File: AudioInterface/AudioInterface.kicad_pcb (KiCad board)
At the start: 2 copper layers, 21 parts, among them J1 Capsule, J2 Set_Gain, J3 Audio_Out, J4 Power, U1 THAT1512, U2 NMA0515SC

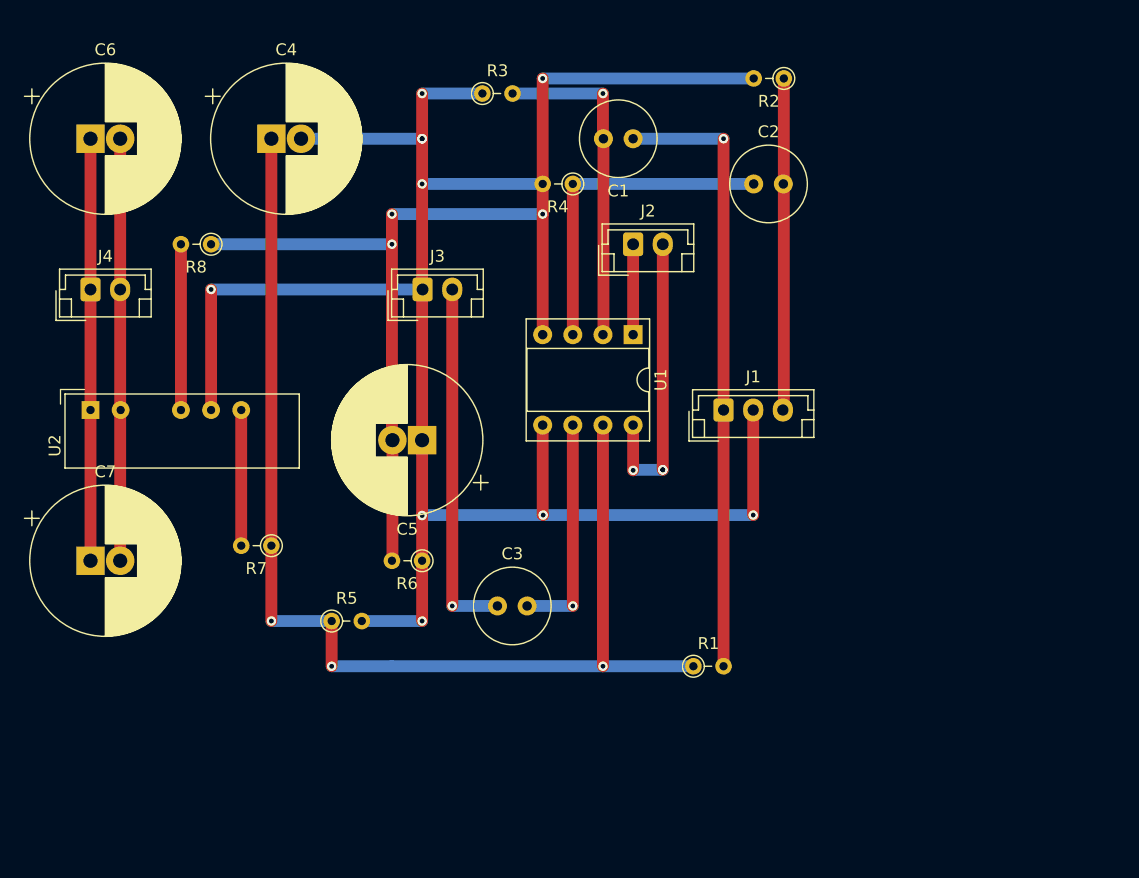
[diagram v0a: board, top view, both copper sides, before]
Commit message: finished pcb
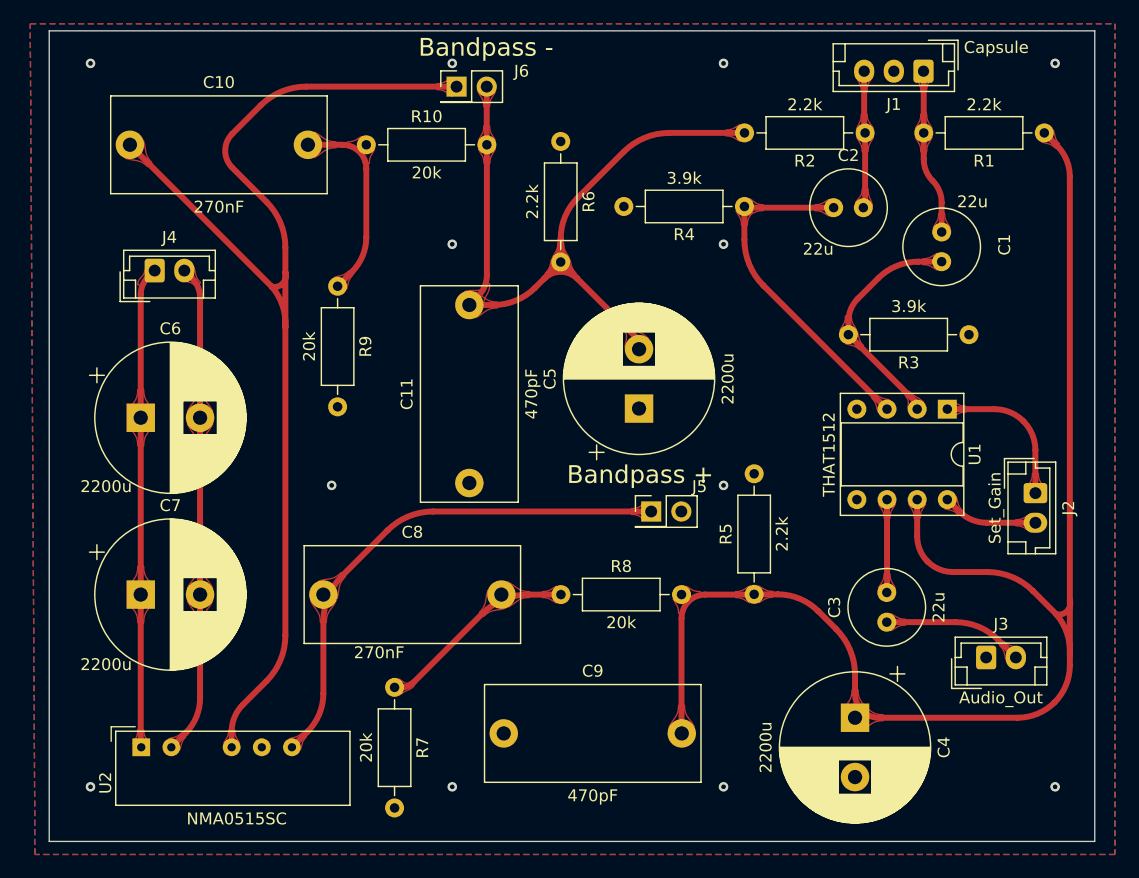
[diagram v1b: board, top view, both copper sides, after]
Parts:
- added C10: 270nF, Capacitor_THT:C_Rect_L18.0mm_W8.0mm_P15.00mm_FKS3_FKP3, F.Cu at (110.0, 60.2)
- added C11: 470pF, Capacitor_THT:C_Rect_L18.0mm_W8.0mm_P15.00mm_FKS3_FKP3, F.Cu at (138.6, 88.7)
- added C8: 270nF, Capacitor_THT:C_Rect_L18.0mm_W8.0mm_P15.00mm_FKS3_FKP3, F.Cu at (126.3, 98.1)
- added C9: 470pF, Capacitor_THT:C_Rect_L18.0mm_W8.0mm_P15.00mm_FKS3_FKP3, F.Cu at (141.5, 109.8)
- added J5: Conn_02x01_Row_Letter_First, Connector_PinHeader_2.54mm:PinHeader_2x01_P2.54mm_Vertical, F.Cu at (153.9, 91.1)
- added J6: Conn_02x01_Row_Letter_First, Connector_PinHeader_2.54mm:PinHeader_2x01_P2.54mm_Vertical, F.Cu at (137.5, 55.3)
- added R10: 20k, Resistor_THT:R_Axial_DIN0207_L6.3mm_D2.5mm_P10.16mm_Horizontal, F.Cu at (129.9, 60.2)
- added R9: 20k, Resistor_THT:R_Axial_DIN0207_L6.3mm_D2.5mm_P10.16mm_Horizontal, F.Cu at (127.5, 72.1)
- C4, C5, C6, C7: footprint Capacitor_THT:CP_Radial_D12.5mm_P2.50mm -> Capacitor_THT:CP_Radial_D12.5mm_P5.00mm
- R1, R2, R3, R4, R5, R6: footprint Resistor_THT:R_Axial_DIN0204_L3.6mm_D1.6mm_P2.54mm_Vertical -> Resistor_THT:R_Axial_DIN0207_L6.3mm_D2.5mm_P10.16mm_Horizontal
- R7, R8: value 100 -> 20k; footprint Resistor_THT:R_Axial_DIN0204_L3.6mm_D1.6mm_P2.54mm_Vertical -> Resistor_THT:R_Axial_DIN0207_L6.3mm_D2.5mm_P10.16mm_Horizontal
- U2: footprint Converter_DCDC:Converter_DCDC_muRata_NMAxxxxSC_THT -> Converter_DCDC:Converter_DCDC_Murata_NMAxxxxSC_THT
- moved C4 69.3 mm to (171.1, 108.5), turned to -90 degrees
- moved J3 56.7 mm to (182.2, 103.4)
- moved R1 53.8 mm to (187.1, 59.2), turned to 180 degrees
- moved R3 45.8 mm to (180.7, 76.2), turned to 180 degrees
- moved R8 41.7 mm to (146.3, 98.1), turned to 0 degrees
- moved J2 39.9 mm to (186.3, 89.5), turned to -90 degrees
- moved R6 37.2 mm to (146.3, 59.9), turned to -90 degrees
- moved R5 35.7 mm to (162.6, 98.1), turned to 90 degrees
- moved J1 33.2 mm to (176.9, 54.0), turned to 180 degrees
- moved C3 32.8 mm to (173.8, 100.4), turned to 90 degrees
- moved U2 28.7 mm to (111.0, 111.0)
- moved U1 27.2 mm to (178.9, 82.5)
- moved C1 27.2 mm to (178.4, 67.5), turned to -90 degrees
- moved C6 23.9 mm to (110.9, 83.2)
- moved C5 18.5 mm to (152.9, 82.4), turned to 90 degrees
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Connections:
- C4 pad 1: Net-(C4-Pad1) -> /Bandpass+/B_OUT
- C5 pad 2: Net-(C5-Pad2) -> /Bandpass-/B_OUT
- R1 pad 1: Net-(C4-Pad1) -> /Bandpass+/B_OUT
- R2 pad 2: Net-(C5-Pad2) -> /Bandpass-/B_OUT
- R5 pad 1: Net-(C4-Pad1) -> /Bandpass+/B_OUT
- R6 pad 2: Net-(C5-Pad2) -> /Bandpass-/B_OUT
- R7 pad 1: Net-(C4-Pad1) -> Net-(C8-Pad2)
- R7 pad 2: Net-(R7-Pad2) -> GND
- R8 pad 1: Net-(C5-Pad2) -> Net-(C8-Pad2)
- R8 pad 2: Net-(R8-Pad2) -> /Bandpass+/B_OUT
- U1 pad 4: Net-(C5-Pad2) -> /Bandpass-/B_OUT
- U1 pad 7: Net-(C4-Pad1) -> /Bandpass+/B_OUT
- U2 pad 4: Net-(R8-Pad2) -> /Bandpass-/B_IN
- U2 pad 6: Net-(R7-Pad2) -> /Bandpass+/B_IN
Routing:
- net GND: track 147.3 -> 0.00 mm, vias 9 -> 12
- net /Bandpass+/B_OUT: track 0.00 -> 121.1 mm
- net Net-(C4-Pad1): track 100.3 -> 0.00 mm, vias 4 -> 0
- net /Bandpass-/B_IN: track 0.00 -> 97.7 mm
- net Net-(C5-Pad2): track 96.6 -> 0.00 mm, vias 4 -> 0
- net /Bandpass-/B_OUT: track 0.00 -> 63.2 mm
- net /Bandpass+/B_IN: track 0.00 -> 43.7 mm
- net Net-(C1-Pad1): track 52.1 -> 14.0 mm, vias 1 -> 0
- net Net-(C3-Pad1): track 30.5 -> 11.9 mm, vias 1 -> 0
- net Net-(J2-Pad2): track 25.3 -> 8.07 mm, vias 3 -> 0
- net Net-(C8-Pad2): track 0.00 -> 16.9 mm
- net Net-(C10-Pad2): track 0.00 -> 16.7 mm
- net Net-(C2-Pad2): track 28.0 -> 11.8 mm
- net Net-(R8-Pad2): track 14.0 -> 0.00 mm
- net Net-(R7-Pad2): track 11.4 -> 0.00 mm
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- added copper zone on B.Cu, net GND
- added copper zone on F.Cu, net GND
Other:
- board outline added: 88.1 x 68.3 mm
- net class Default removed
- board text added: "Bandpass +"
- board text added: "Bandpass -"
